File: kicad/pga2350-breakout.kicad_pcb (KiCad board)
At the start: 2 copper layers, 50.8 x 41.9 mm, 5 parts, among them J1 Conn_01x02_Pin, J2 Conn_02x05_Odd_Even, J3 Conn_01x02_Pin, J4 Conn_01x05_Pin

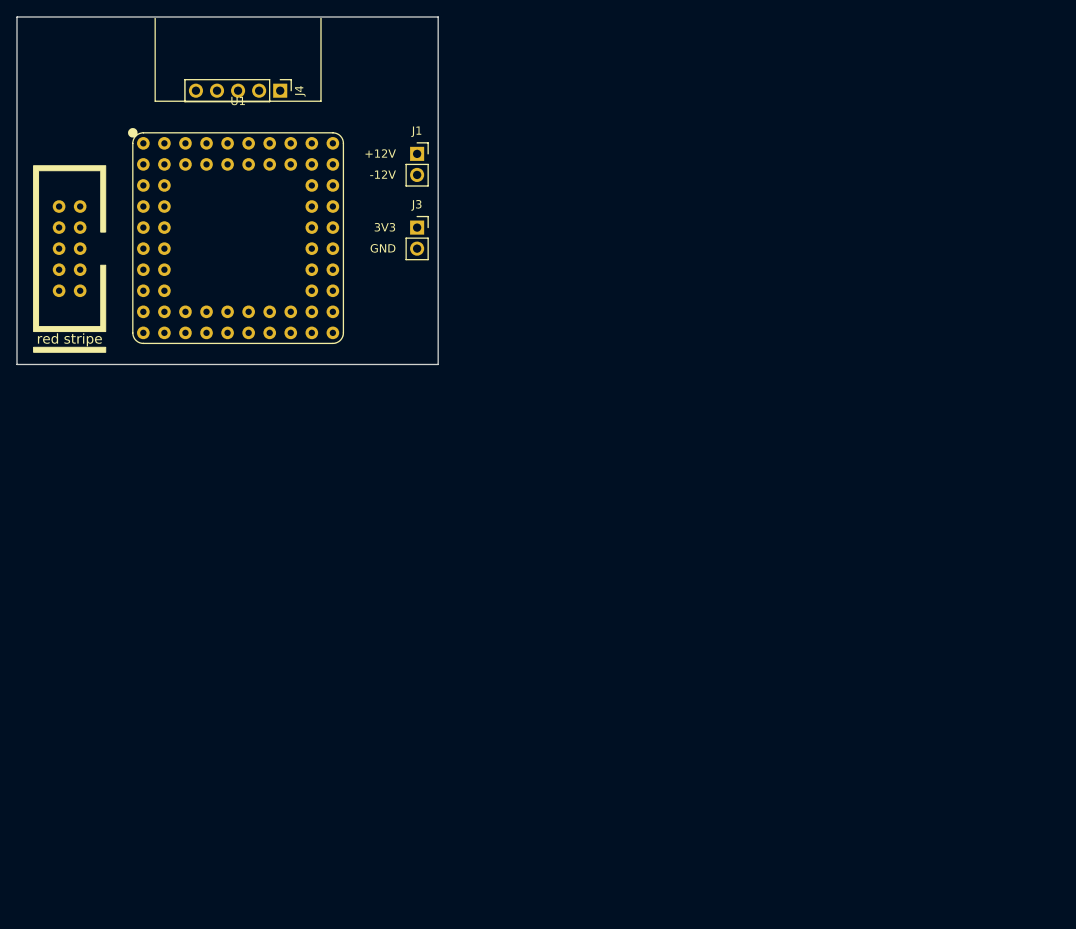
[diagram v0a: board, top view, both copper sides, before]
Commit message: initial routing, DRC all clear
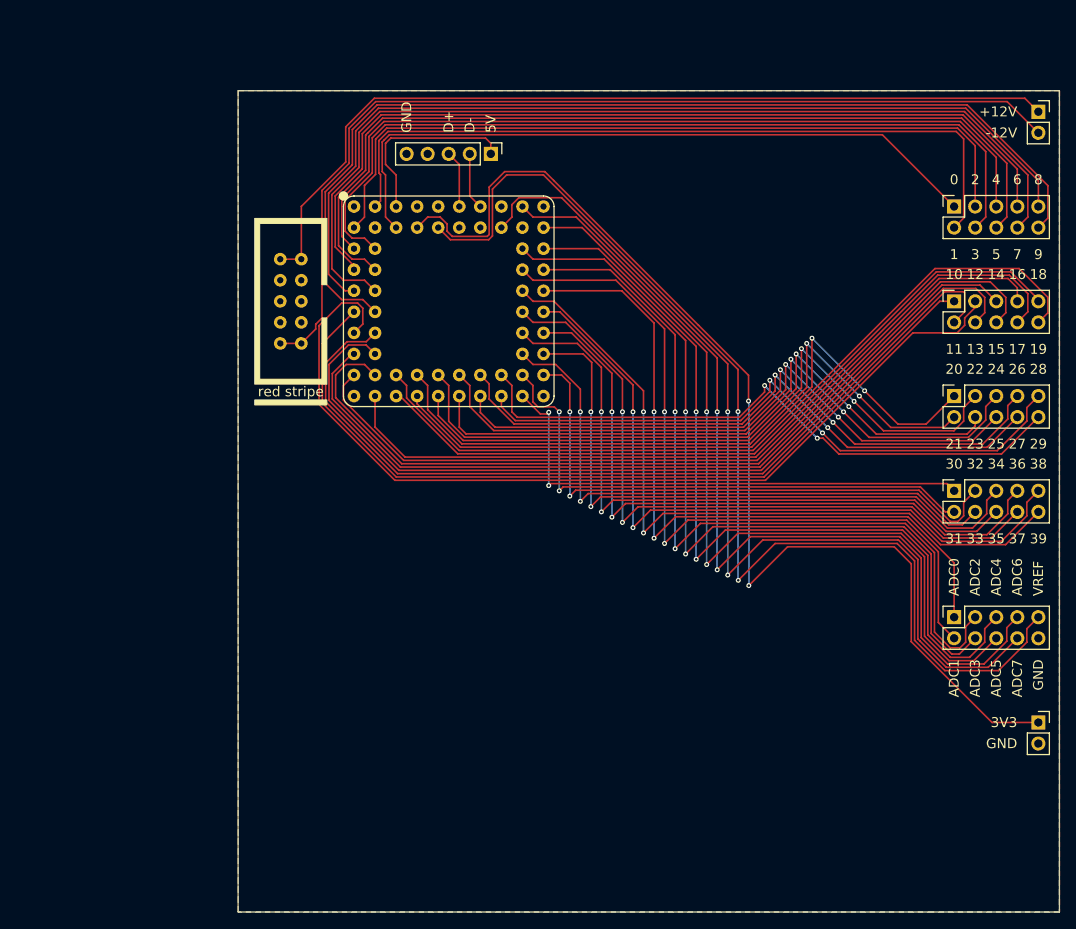
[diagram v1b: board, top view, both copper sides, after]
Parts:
- added J10: Conn_02x05_Counter_Clockwise, Connector_PinSocket_2.54mm:PinSocket_2x05_P2.54mm_Vertical, F.Cu at (86.4, 14.0)
- added J5: Conn_02x05_Counter_Clockwise, Connector_PinSocket_2.54mm:PinSocket_2x05_P2.54mm_Vertical, F.Cu at (86.4, 25.4)
- added J6: Conn_02x05_Counter_Clockwise, Connector_PinSocket_2.54mm:PinSocket_2x05_P2.54mm_Vertical, F.Cu at (86.4, 36.8)
- added J7: Conn_02x05_Counter_Clockwise, Connector_PinSocket_2.54mm:PinSocket_2x05_P2.54mm_Vertical, F.Cu at (86.4, 48.3)
- added J8: Conn_02x05_Counter_Clockwise, Connector_PinSocket_2.54mm:PinSocket_2x05_P2.54mm_Vertical, F.Cu at (86.4, 63.5)
- moved J3 95.8 mm to (96.5, 76.2)
- moved J1 75.1 mm to (96.5, 2.54)
- moved J2 27.4 mm to (6.36, 25.4)
- moved J4 26.5 mm to (30.5, 7.62)
- moved U1 26.5 mm to (25.4, 25.4)
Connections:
- J2 pad 3: Net-(J2-Pin_3) -> GND
- J2 pad 4: Net-(J2-Pin_3) -> GND
- J2 pad 7: Net-(J2-Pin_7) -> GND
- J2 pad 8: Net-(J2-Pin_7) -> GND
- U1 pad 10: unconnected-(U1-GP10-Pad10) -> /GP10
- U1 pad 11: unconnected-(U1-GP11-Pad11) -> /GP11
- U1 pad 12: unconnected-(U1-GP12-Pad12) -> /GP12
- U1 pad 13: unconnected-(U1-GP13-Pad13) -> /GP13
- U1 pad 14: unconnected-(U1-GP14-Pad14) -> /GP14
- U1 pad 15: unconnected-(U1-GP15-Pad15) -> /GP15
- U1 pad 16: unconnected-(U1-GP16-Pad16) -> /GP16
- U1 pad 17: unconnected-(U1-GP17-Pad17) -> /GP17
- U1 pad 19: unconnected-(U1-GP18-Pad19) -> /GP18
- U1 pad 2: unconnected-(U1-GP2-Pad2) -> /GP2
- U1 pad 20: unconnected-(U1-GP19-Pad20) -> /GP19
- U1 pad 21: unconnected-(U1-GP20-Pad21) -> /GP20
- U1 pad 22: unconnected-(U1-GP21-Pad22) -> /GP21
- U1 pad 23: unconnected-(U1-GP22-Pad23) -> /GP22
- U1 pad 24: unconnected-(U1-GP23-Pad24) -> /GP23
- U1 pad 25: unconnected-(U1-GP24-Pad25) -> /GP24
- U1 pad 26: unconnected-(U1-GP25-Pad26) -> /GP25
- U1 pad 27: unconnected-(U1-GP26-Pad27) -> /GP26
- U1 pad 28: unconnected-(U1-GP27-Pad28) -> /GP27
- U1 pad 29: unconnected-(U1-GP28-Pad29) -> /GP28
- U1 pad 3: unconnected-(U1-GP3-Pad3) -> /GP3
- U1 pad 30: unconnected-(U1-GP29-Pad30) -> /GP29
- U1 pad 31: unconnected-(U1-GP30-Pad31) -> /GP30
- U1 pad 32: unconnected-(U1-GP31-Pad32) -> /GP31
- U1 pad 34: unconnected-(U1-GP32-Pad34) -> /GP32
- U1 pad 35: unconnected-(U1-GP33-Pad35) -> /GP33
- U1 pad 36: unconnected-(U1-GP34-Pad36) -> /GP34
- U1 pad 37: unconnected-(U1-GP35-Pad37) -> /GP35
- U1 pad 38: unconnected-(U1-GP36-Pad38) -> /GP36
- U1 pad 39: unconnected-(U1-GP37-Pad39) -> /GP37
- U1 pad 4: unconnected-(U1-GP4-Pad4) -> /GP4
- U1 pad 40: unconnected-(U1-GP38-Pad40) -> /GP38
- U1 pad 41: unconnected-(U1-GP39-Pad41) -> /GP39
- U1 pad 42: unconnected-(U1-GP40-Pad42) -> /GP40
- U1 pad 43: unconnected-(U1-GP41-Pad43) -> /GP41
- U1 pad 44: unconnected-(U1-GP42-Pad44) -> /GP42
- U1 pad 45: unconnected-(U1-GP43-Pad45) -> /GP43
- U1 pad 46: unconnected-(U1-GP44-Pad46) -> /GP44
- U1 pad 47: unconnected-(U1-GP45-Pad47) -> /GP45
- U1 pad 49: unconnected-(U1-GP46-Pad49) -> /GP46
- U1 pad 5: unconnected-(U1-GP5-Pad5) -> /GP5
- U1 pad 50: unconnected-(U1-GP47-Pad50) -> /GP47
- U1 pad 51: unconnected-(U1-BOOTSEL-Pad51) -> /BOOTSETL
- U1 pad 52: unconnected-(U1-SWDIO-Pad52) -> /SWDIO
- U1 pad 55: unconnected-(U1-SWCLK-Pad55) -> /SWCLK
- U1 pad 56: unconnected-(U1-RUN-Pad56) -> /RUN
- U1 pad 57: unconnected-(U1-ADC_VREF-Pad57) -> /ADC_VREF
- U1 pad 58: unconnected-(U1-3V3_EN-Pad58) -> /3V3_EN
- U1 pad 6: unconnected-(U1-GP6-Pad6) -> /GP6
- U1 pad 61: unconnected-(U1-GP0-Pad61) -> /GP0
- U1 pad 62: unconnected-(U1-GP1-Pad62) -> /GP1
- U1 pad 7: unconnected-(U1-GP7-Pad7) -> /GP7
- U1 pad 8: unconnected-(U1-GP8-Pad8) -> /GP8
- U1 pad 9: unconnected-(U1-GP9-Pad9) -> /GP9
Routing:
- net +3V3: track 0.00 -> 135.3 mm, vias 0 -> 2
- net /ADC_VREF: track 0.00 -> 132.1 mm, vias 0 -> 2
- net /GP9: track 0.00 -> 122.0 mm
- net -12V: track 0.00 -> 116.9 mm
- net /GP7: track 0.00 -> 115.9 mm
- net /GP47: track 0.00 -> 113.5 mm, vias 0 -> 2
- net /GP8: track 0.00 -> 112.7 mm
- net /GP12: track 0.00 -> 112.4 mm
- net /GP46: track 0.00 -> 109.7 mm, vias 0 -> 2
- net /GP5: track 0.00 -> 109.0 mm
- net /GP13: track 0.00 -> 106.9 mm
- net +12V: track 0.00 -> 106.4 mm
- net /GP15: track 0.00 -> 106.0 mm
- net /GP11: track 0.00 -> 106.0 mm
- net /GP6: track 0.00 -> 106.0 mm
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- added copper zone on B.Cu, net GND
- added copper zone on F.Cu, net GND
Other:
- board size 50.8 x 41.9 mm -> 99.1 x 99.1 mm
- board text added: "0"
- board text added: "1"
- board text added: "10"
- board text added: "11"
- board text added: "12"
- board text added: "13"
- board text added: "14"
- board text added: "15"
- board text added: "16"
- board text added: "17"
- board text added: "18"
- board text added: "19"
- board text added: "2"
- board text added: "20"
- board text added: "21"
- board text added: "22"
- board text added: "23"
- board text added: "24"
- board text added: "25"
- board text added: "26"
- board text added: "27"
- board text added: "28"
- board text added: "29"
- board text added: "3"
- board text added: "30"
- board text added: "31"
- board text added: "32"
- board text added: "33"
- board text added: "34"
- board text added: "35"
- board text added: "36"
- board text added: "37"
- board text added: "38"
- board text added: "39"
- board text added: "4"
- board text added: "5"
- board text added: "5V"
- board text added: "6"
- board text added: "7"
- board text added: "8"
- board text added: "9"
- board text added: "ADC0"
- board text added: "ADC1"
- board text added: "ADC2"
- board text added: "ADC3"
- board text added: "ADC4"
- board text added: "ADC5"
- board text added: "ADC6"
- board text added: "ADC7"
- board text added: "D+"
- board text added: "D-"
- board text added: "VREF"
